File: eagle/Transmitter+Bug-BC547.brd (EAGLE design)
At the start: 27.9 x 20.3 mm, 14 parts, among them T1 BC547

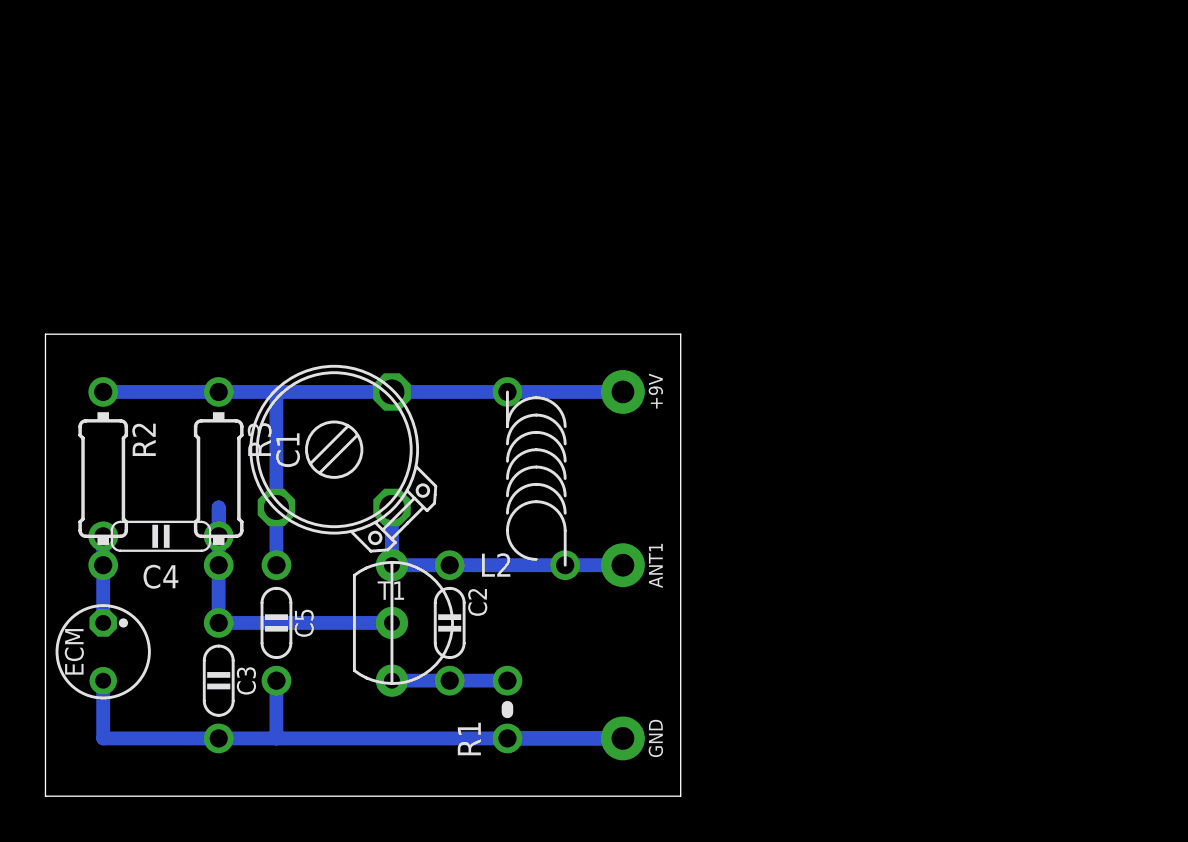
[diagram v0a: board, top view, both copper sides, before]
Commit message: ...
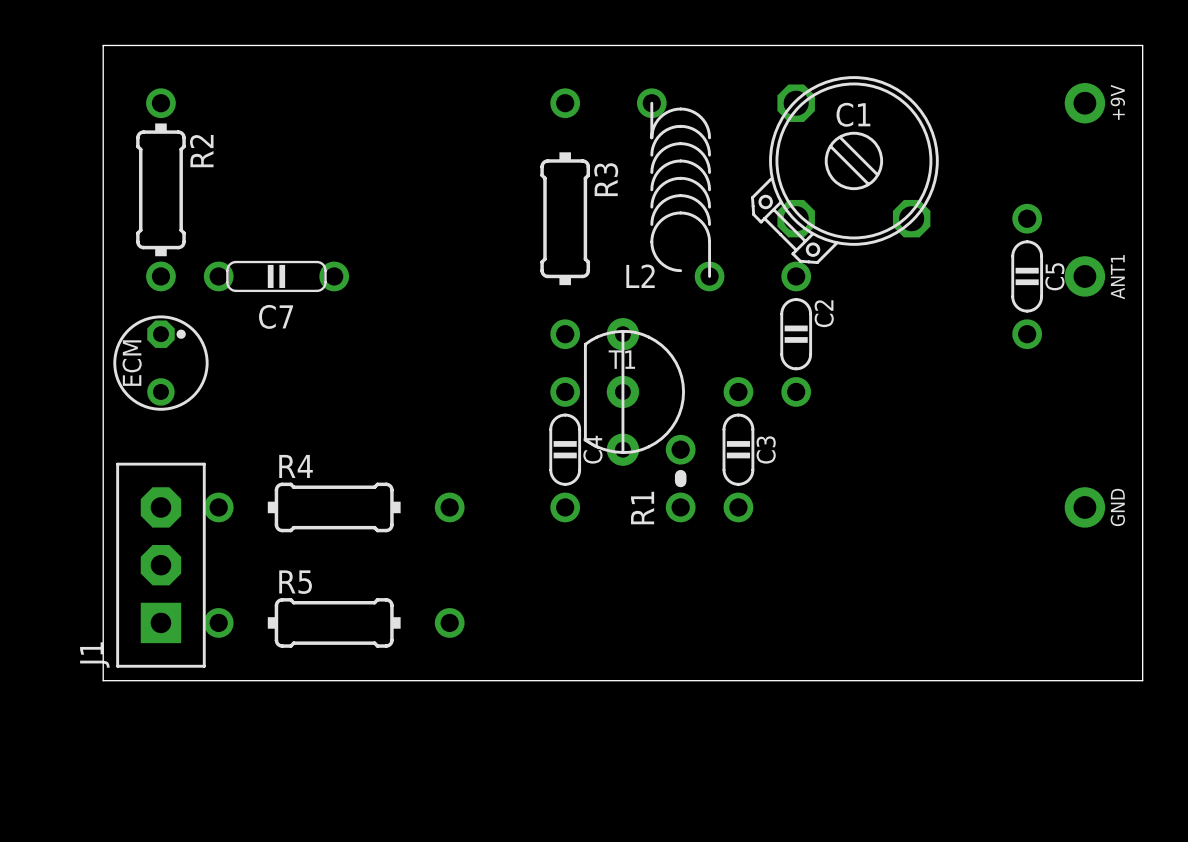
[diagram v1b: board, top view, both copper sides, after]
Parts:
- added C7: 330nF, c:C050-020X044
- added J1: CONN-3P-3P, pinconn:CONN-3P
- added R4, R5: 22k, r:0204/10
- C4: value 330nF -> 1nF; device c:C050-020X044 -> c:C050-020X036/V
- R3: device r:0204/7-V -> r:0204/10-V
- moved C5 36.4 mm to (43.2, 22.9)
- moved C1 26.2 mm to (35.6, 27.9), turned to 0 degrees
- moved C3 25.0 mm to (30.5, 15.2)
- moved +9V 24.0 mm to (45.7, 30.5)
- moved ANT1 24.0 mm to (45.7, 22.9)
- moved GND 22.7 mm to (45.7, 12.7)
- moved C2 19.8 mm to (33.0, 20.3)
- moved R3 19.0 mm to (22.9, 25.4)
- moved C4 18.2 mm to (22.9, 15.2)
- moved T1 14.4 mm to (25.4, 17.8)
- moved L2 14.2 mm to (27.9, 27.9)
- moved ECM 13.0 mm to (5.08, 19.1)
- moved R2 13.0 mm to (5.08, 26.7)
- moved R1 12.7 mm to (27.9, 14.0)
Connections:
- removed net N$5: C3.1, C4.2, R3.1, T1.B
- new net MOD: C4.1, C7.2, R3.1, R4.2, R5.2, T1.B
- new net N$1: J1.3, R4.1
- new net N$4: J1.1, R5.1
- net +UB: no longer C1.3
- net GND: now also C4.2, J1.2
- net N$3: now also C3.1
- net N$6: now also C7.1; no longer C4.1
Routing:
- net GND: track 33.0 -> 0.00 mm
- net +UB: track 30.5 -> 0.00 mm
- net N$5: track 14.0 -> 0.00 mm
- net N$2: track 12.7 -> 0.00 mm
- net N$3: track 5.08 -> 0.00 mm
- net N$6: track 3.81 -> 0.00 mm
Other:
- board size 27.9 x 20.3 mm -> 45.7 x 27.9 mm

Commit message: ...
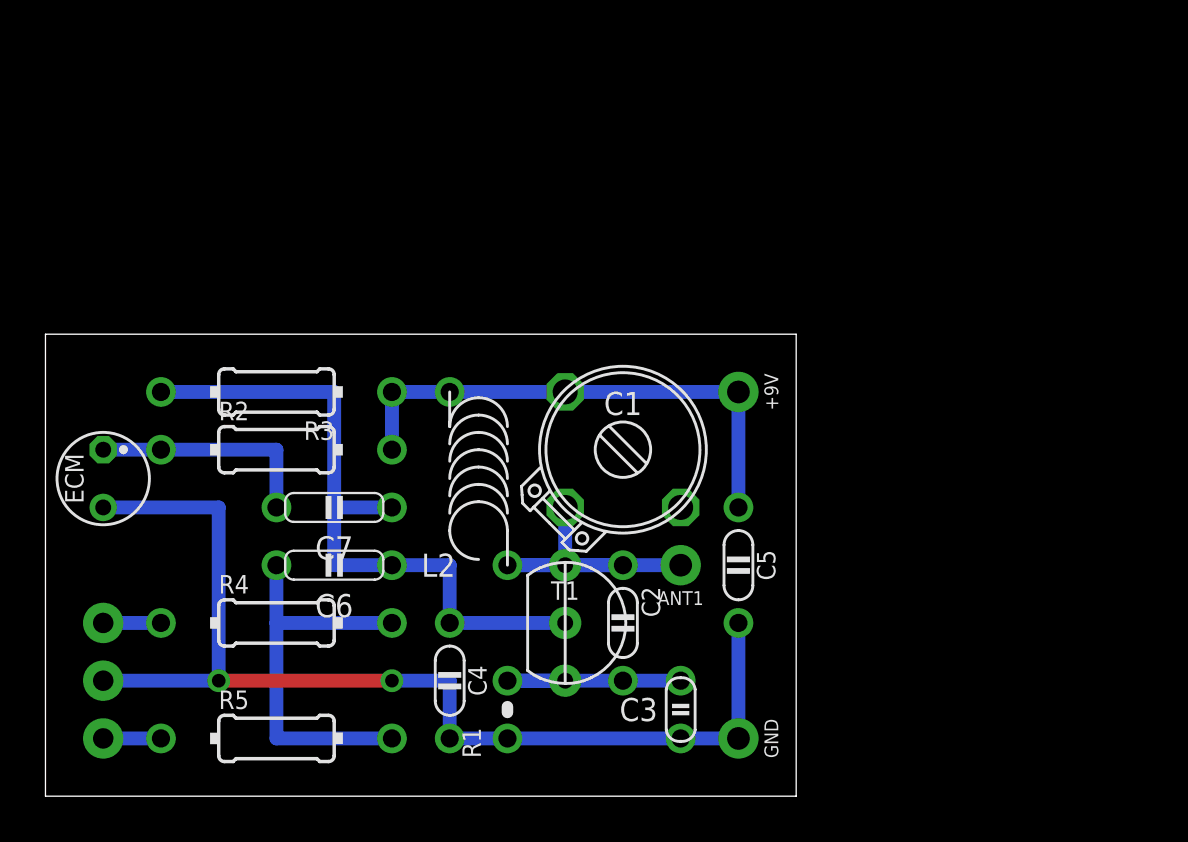
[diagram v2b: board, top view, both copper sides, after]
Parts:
- removed J1: CONN-3P-3P, pinconn:CONN-3P
- added C6: 330nF, c:C050-020X044
- added J2: SAUDIO, pad:SPAD-3
- C3: device c:C050-020X036/V -> c:C025-015X024
- R2: device r:0204/7-V -> r:0204/10
- moved ANT1 21.8 mm to (27.9, 10.2), turned to 90 degrees
- moved +9V 19.8 mm to (30.5, 17.8)
- moved GND 18.3 mm to (30.5, 2.54)
- moved C5 18.0 mm to (30.5, 10.2)
- moved C1 16.3 mm to (25.4, 15.2)
- moved L2 15.5 mm to (19.1, 15.2)
- moved C2 14.8 mm to (25.4, 7.62)
- moved R3 14.8 mm to (10.2, 17.8), turned to 90 degrees
- moved R1 12.7 mm to (20.3, 3.81)
- moved R2 12.5 mm to (10.2, 15.2), turned to 0 degrees
- moved C3 11.7 mm to (27.9, 3.81), turned to 0 degrees
- moved C4 11.4 mm to (17.8, 5.08)
- moved C7 10.5 mm to (12.7, 12.7)
- moved T1 10.5 mm to (22.9, 7.62)
- moved ECM 5.68 mm to (2.54, 14.0)
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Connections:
- new net N$5: C6.1, R4.2, R5.2
- net GND: now also J2.2; no longer J1.2
- net MOD: now also C6.2; no longer R4.2, R5.2
- net N$1: now also J2.1; no longer J1.3
- net N$4: now also J2.3; no longer J1.1
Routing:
- net GND: track 0.00 -> 48.3 mm, vias 0 -> 2
- net MOD: track 0.00 -> 30.5 mm
- net +UB: track 0.00 -> 22.9 mm
- net N$5: track 0.00 -> 17.8 mm
- net N$2: track 0.00 -> 15.2 mm
- net N$6: track 0.00 -> 10.2 mm
- net N$3: track 0.00 -> 10.2 mm
- net N$4: track 0.00 -> 2.54 mm
- net N$1: track 0.00 -> 2.54 mm
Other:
- board size 45.7 x 27.9 mm -> 33 x 20.3 mm

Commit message: ...
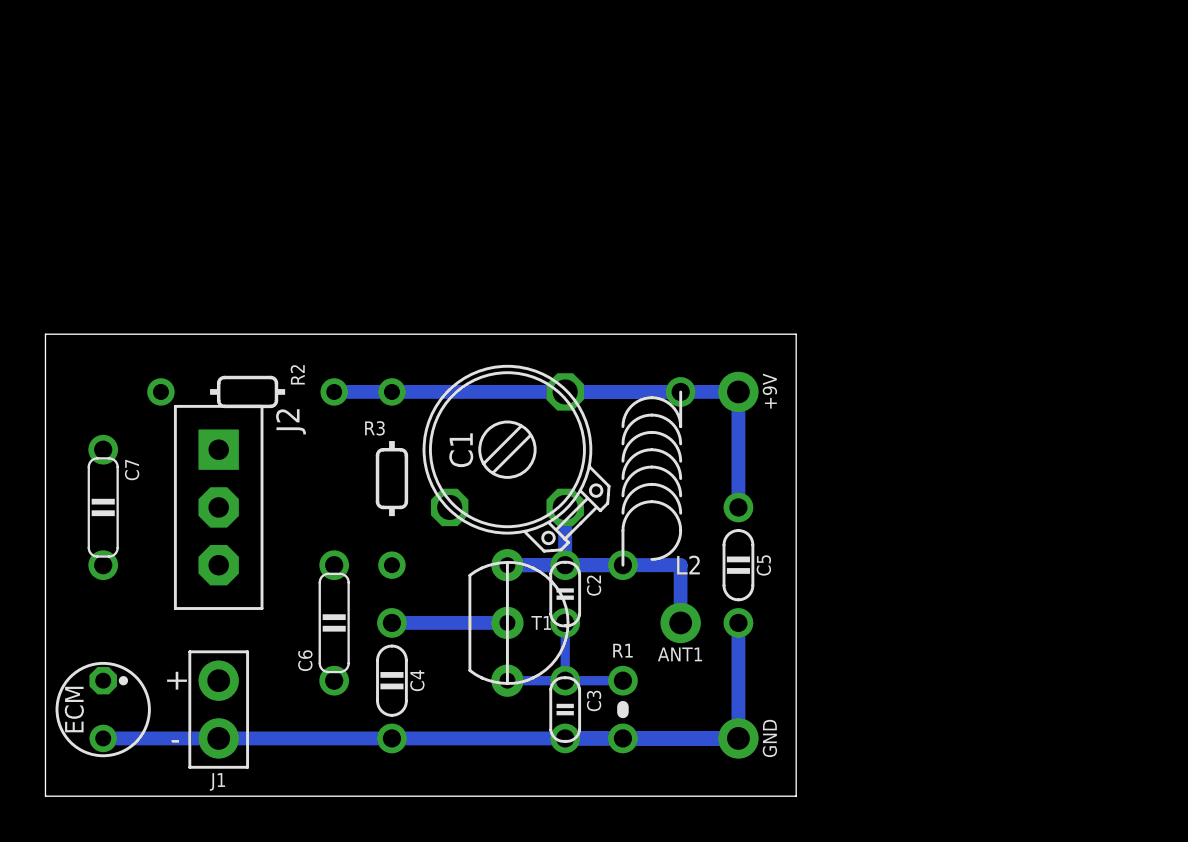
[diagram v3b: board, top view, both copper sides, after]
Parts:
- removed R4, R5: 22k, r:0204/10
- added J1: (no value), pad:SPAD-+
- C2: device c:C050-020X036 -> c:C025-015X024
- J2: value SAUDIO -> (none); device pad:SPAD-3 -> pinconn:CONN-3P
- L2: device l:L-04/7V -> l:L-04/7V-X
- R2: device r:0204/10 -> r:0202/7-V
- R3: device r:0204/10-V -> r:0202/7-V
- moved J2 11.4 mm to (7.62, 15.2)
- moved C7 10.2 mm to (2.54, 12.7), turned to 270 degrees
- moved ECM 10.2 mm to (2.54, 3.81)
- moved L2 7.73 mm to (26.7, 14.0)
- moved R3 6.35 mm to (15.2, 14.0), turned to 0 degrees
- moved C3 5.08 mm to (22.9, 3.81), turned to 270 degrees
- moved C1 5.08 mm to (20.3, 15.2), turned to 90 degrees
- moved R1 5.08 mm to (25.4, 3.81), turned to 0 degrees
- moved R2 2.84 mm to (8.89, 17.8), turned to 270 degrees
- moved C2 2.84 mm to (22.9, 8.89)
- moved C4 2.54 mm to (15.2, 5.08)
- moved ANT1 2.54 mm to (27.9, 7.62)
- moved C6 2.54 mm to (12.7, 7.62), turned to 90 degrees
- moved T1 2.54 mm to (20.3, 7.62)
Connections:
- net +UB: now also C1.3, R2.1, R3.1; no longer C1.1, R2.2, R3.2
- net GND: now also J1.1, R1.2; no longer J2.2, R1.1
- net MOD: now also J2.2, R3.2; no longer C6.2, C7.2, R3.1
- net N$1: now also C6.2, J2.3; no longer J2.1, R4.1
- net N$3: now also R1.1; no longer R1.2
- net N$4: now also C7.2, J2.1; no longer J2.3, R5.1
- net N$5: now also J1.2; no longer R4.2, R5.2
- net N$6: now also R2.2; no longer R2.1
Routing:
- net MOD: track 30.5 -> 5.08 mm
- net N$5: track 17.8 -> 0.00 mm
- net +UB: track 22.9 -> 33.0 mm
- net N$6: track 10.2 -> 0.00 mm
- net N$3: track 10.2 -> 7.62 mm
- net N$4: track 2.54 -> 0.00 mm
- net N$1: track 2.54 -> 0.00 mm
- net N$2: track 15.2 -> 17.8 mm
- net GND: track 48.3 -> 45.7 mm, vias 2 -> 0

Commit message: ...
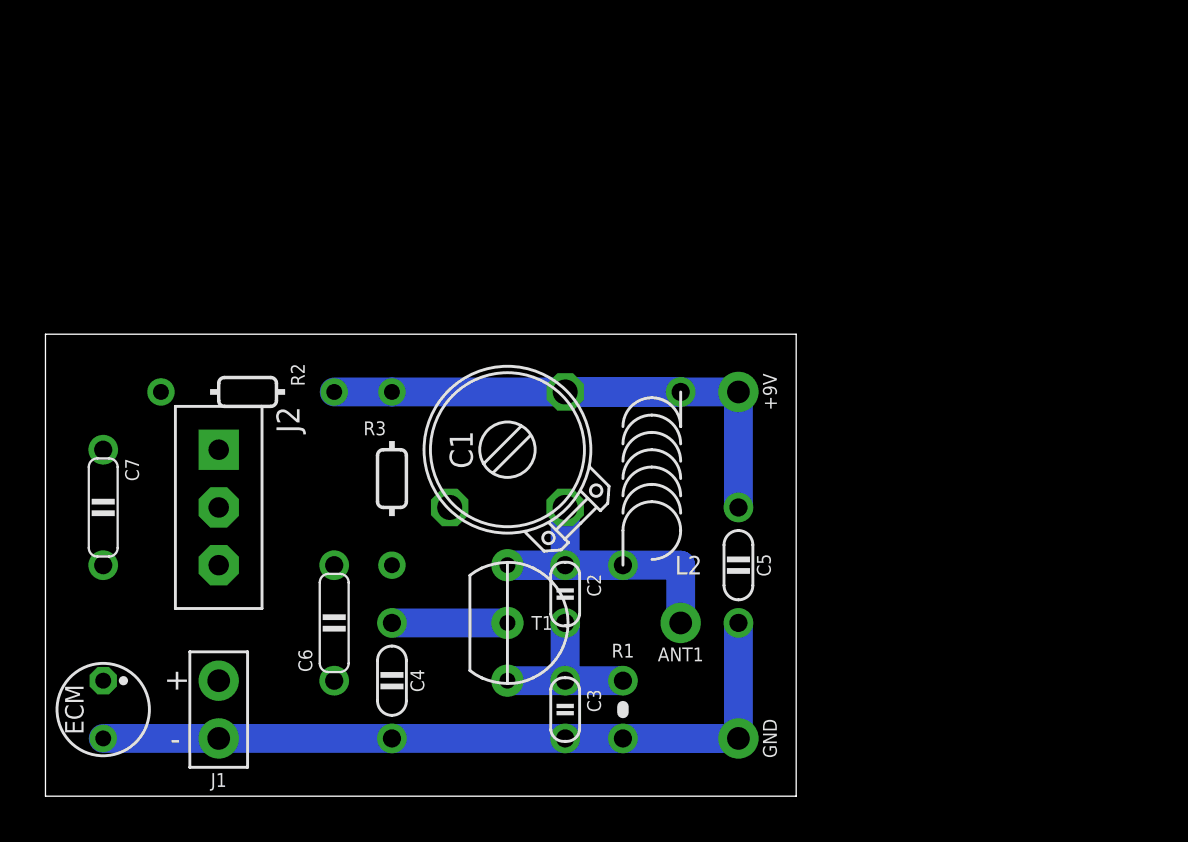
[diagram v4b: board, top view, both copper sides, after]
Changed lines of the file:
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@@
 <contactref element="C3" pad="1"/>
 <wire x1="22.86" y1="5.08" x2="25.4" y2="5.08" width="0" layer="19" extent="1-1"/>
-<wire x1="25.4" y1="5.08" x2="22.86" y2="5.08" width="0.4064" layer="16"/>
-<wire x1="22.86" y1="5.08" x2="22.86" y2="7.62" width="0.4064" layer="16"/>
-<wire x1="20.32" y1="5.08" x2="22.86" y2="5.08" width="0.4064" layer="16"/>
+<wire x1="25.4" y1="5.08" x2="22.86" y2="5.08" width="1.27" layer="16"/>
+<wire x1="22.86" y1="5.08" x2="22.86" y2="7.62" width="1.27" layer="16"/>
+<wire x1="20.32" y1="5.08" x2="22.86" y2="5.08" width="1.27" layer="16"/>
 </signal>
 <signal name="N$6">
@@
 <contactref element="ECM" pad="2"/>
 <contactref element="C3" pad="2"/>
-<wire x1="2.54" y1="2.54" x2="7.62" y2="2.54" width="0.6096" layer="16"/>
-<wire x1="7.62" y1="2.54" x2="15.24" y2="2.54" width="0.6096" layer="16"/>
-<wire x1="30.48" y1="2.54" x2="15.24" y2="2.54" width="0.6096" layer="16"/>
-<wire x1="30.48" y1="7.62" x2="30.48" y2="2.54" width="0.6096" layer="16"/>
-<wire x1="22.86" y1="2.54" x2="30.48" y2="2.54" width="0.6096" layer="16"/>
-<wire x1="30.48" y1="2.54" x2="25.4" y2="2.54" width="0.6096" layer="16"/>
+<wire x1="2.54" y1="2.54" x2="7.62" y2="2.54" width="1.27" layer="16"/>
+<wire x1="7.62" y1="2.54" x2="15.24" y2="2.54" width="1.27" layer="16"/>
+<wire x1="30.48" y1="2.54" x2="15.24" y2="2.54" width="1.27" layer="16"/>
+<wire x1="30.48" y1="7.62" x2="30.48" y2="2.54" width="1.27" layer="16"/>
+<wire x1="22.86" y1="2.54" x2="30.48" y2="2.54" width="1.27" layer="16"/>
+<wire x1="30.48" y1="2.54" x2="25.4" y2="2.54" width="1.27" layer="16"/>
 <contactref element="J1" pad="1"/>
 </signal>
@@
 <contactref element="L2" pad="2"/>
 <contactref element="R2" pad="1"/>
-<wire x1="22.86" y1="17.78" x2="27.94" y2="17.78" width="0.6096" layer="16"/>
-<wire x1="30.48" y1="12.7" x2="30.48" y2="17.78" width="0.6096" layer="16"/>
-<wire x1="30.48" y1="17.78" x2="22.86" y2="17.78" width="0.6096" layer="16"/>
-<wire x1="27.94" y1="17.78" x2="15.24" y2="17.78" width="0.6096" layer="16"/>
-<wire x1="12.7" y1="17.78" x2="15.24" y2="17.78" width="0.6096" layer="16"/>
+<wire x1="22.86" y1="17.78" x2="27.94" y2="17.78" width="1.27" layer="16"/>
+<wire x1="30.48" y1="12.7" x2="30.48" y2="17.78" width="1.27" layer="16"/>
+<wire x1="30.48" y1="17.78" x2="22.86" y2="17.78" width="1.27" layer="16"/>
+<wire x1="27.94" y1="17.78" x2="15.24" y2="17.78" width="1.27" layer="16"/>
+<wire x1="12.7" y1="17.78" x2="15.24" y2="17.78" width="1.27" layer="16"/>
 </signal>
 <signal name="N$2">
@@
 <contactref element="ANT1" pad="1"/>
 <contactref element="C1" pad="2"/>
-<wire x1="25.4" y1="10.16" x2="20.32" y2="10.16" width="0.6096" layer="16"/>
-<wire x1="20.32" y1="10.16" x2="22.86" y2="10.16" width="0.6096" layer="16"/>
-<wire x1="22.86" y1="10.16" x2="22.86" y2="12.7" width="0.6096" layer="16"/>
-<wire x1="27.94" y1="7.62" x2="27.94" y2="10.16" width="0.6096" layer="16"/>
-<wire x1="27.94" y1="10.16" x2="25.4" y2="10.16" width="0.6096" layer="16"/>
-<wire x1="25.4" y1="10.16" x2="22.86" y2="10.16" width="0.6096" layer="16"/>
+<wire x1="25.4" y1="10.16" x2="20.32" y2="10.16" width="1.27" layer="16"/>
+<wire x1="20.32" y1="10.16" x2="22.86" y2="10.16" width="1.27" layer="16"/>
+<wire x1="22.86" y1="10.16" x2="22.86" y2="12.7" width="1.27" layer="16"/>
+<wire x1="27.94" y1="7.62" x2="27.94" y2="10.16" width="1.27" layer="16"/>
+<wire x1="27.94" y1="10.16" x2="25.4" y2="10.16" width="1.27" layer="16"/>
+<wire x1="25.4" y1="10.16" x2="22.86" y2="10.16" width="1.27" layer="16"/>
 </signal>
 <signal name="MOD">
@@
 <contactref element="C4" pad="1"/>
 <contactref element="T1" pad="B"/>
-<wire x1="20.32" y1="7.62" x2="15.24" y2="7.62" width="0.6096" layer="16"/>
+<wire x1="20.32" y1="7.62" x2="15.24" y2="7.62" width="1.27" layer="16"/>
 <contactref element="J2" pad="2"/>
 <wire x1="15.24" y1="7.62" x2="15.24" y2="10.16" width="0" layer="19" extent="1-1"/>
